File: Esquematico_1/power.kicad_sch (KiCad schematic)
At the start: 13 parts, among them U6 TPS54302DDCR, U7 AP2112K-3.3TRG1

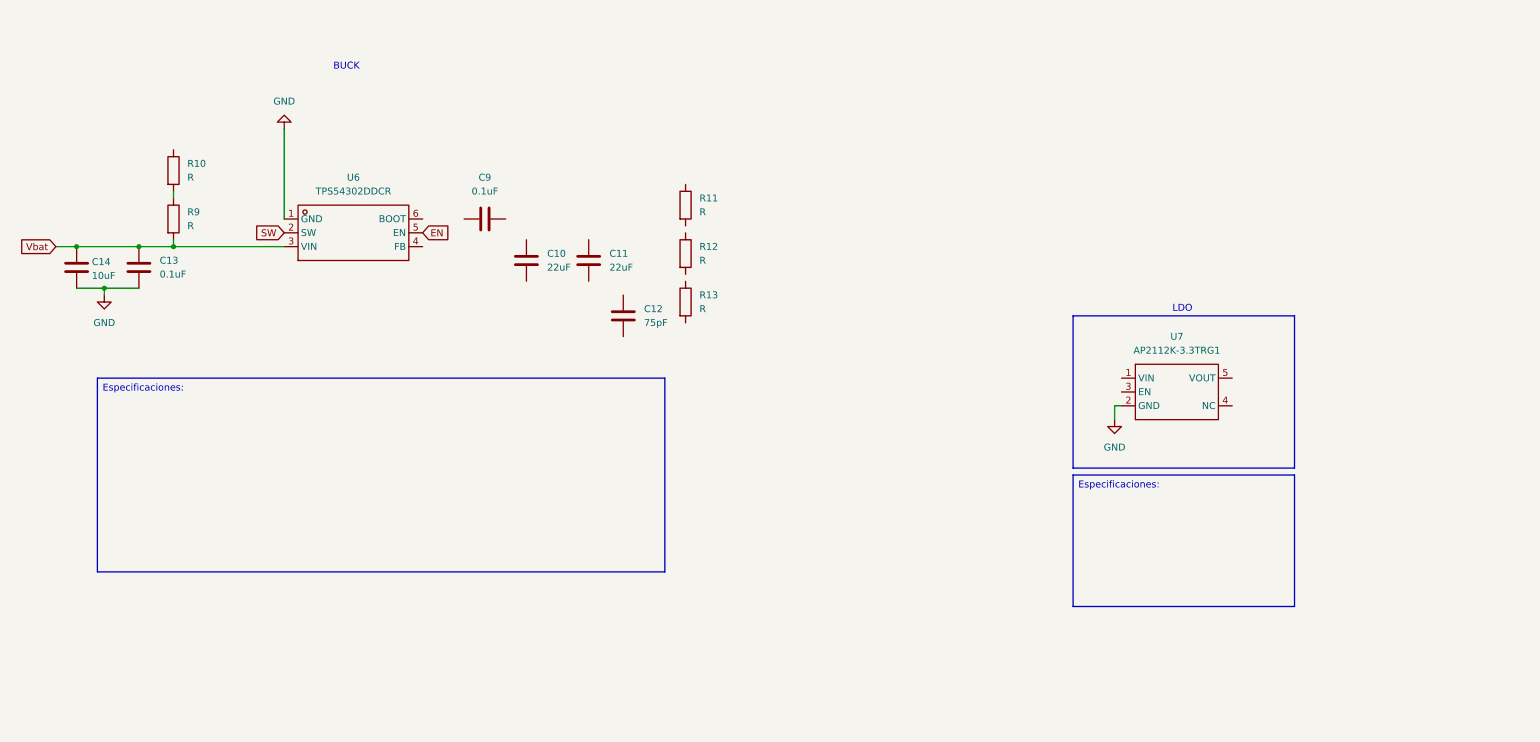
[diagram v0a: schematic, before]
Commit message: Update power
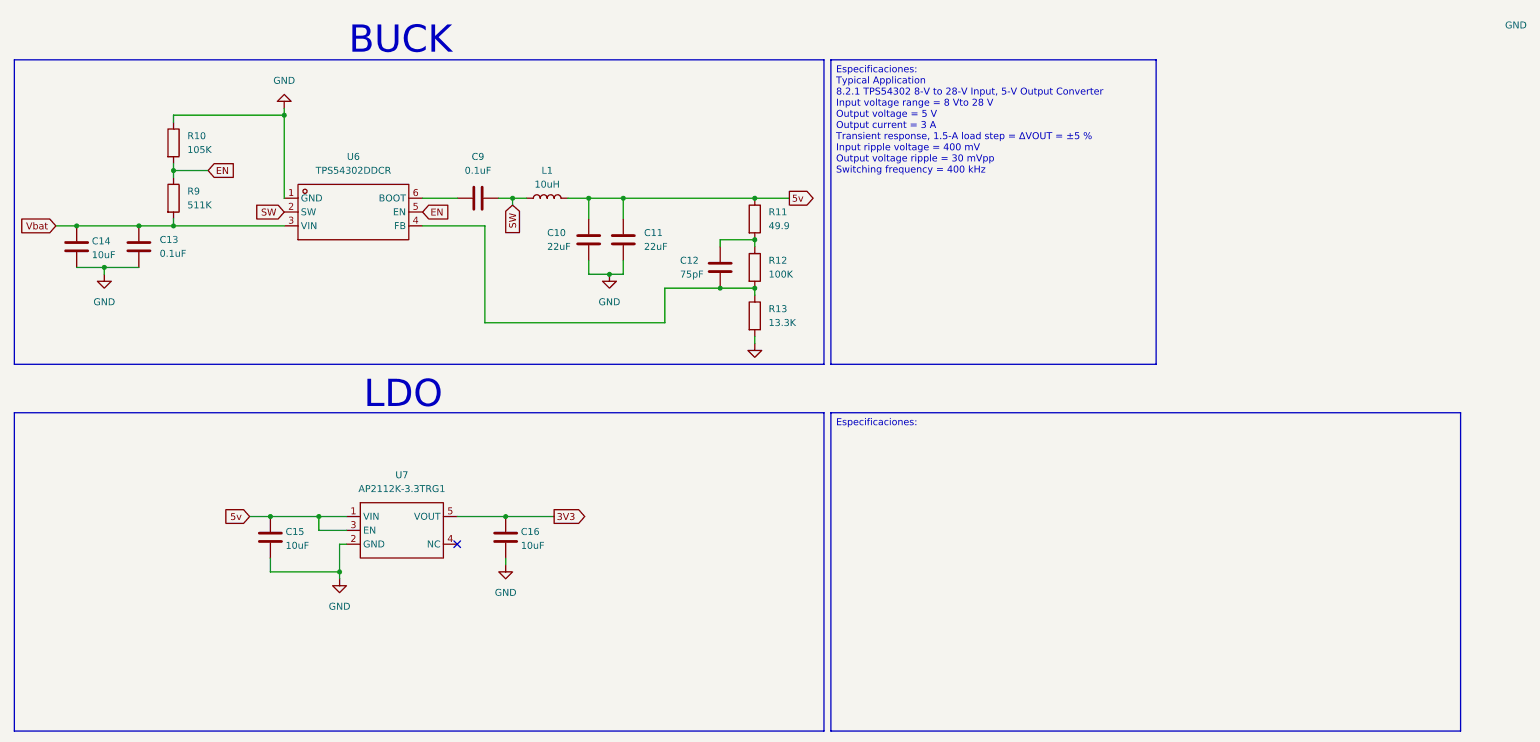
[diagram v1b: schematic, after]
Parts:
- added C15, C16: 10uF, symbol Device:C
- added L1: 10uH, symbol Device:L
- R10: value R -> 105K
- R11: value R -> 49.9
- R12: value R -> 100K
- R13: value R -> 13.3K
- R9: value R -> 511K
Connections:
- net EN: now also R10.2, R9.1
- net GND: now also C10.1, C11.1, R10.1, R13.2, C15.1, C16.1
- net SW: now also C9.2, L1.1
- net at R12.1: now also C12.1, R11.2
- net at R12.2: now also C12.2, R13.1, U6.4 (FB)
- net 5v: now reaches C11.2
- net 5v: now also C10.2, R11.1, U7.1 (VIN), U7.3 (EN), C15.2, L1.2
- net at U6.6 (BOOT): now also C9.1
- net 3V3: now reaches U7.5 (VOUT)
- net 3V3: now also C16.2
- no-connect marks 0 -> 1
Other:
- moved on the sheet: C10, C11, C12, C13, C14, C9, R10, R11, R12, R13, R9, U6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
